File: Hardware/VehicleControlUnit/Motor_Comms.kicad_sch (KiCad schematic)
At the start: 47 parts

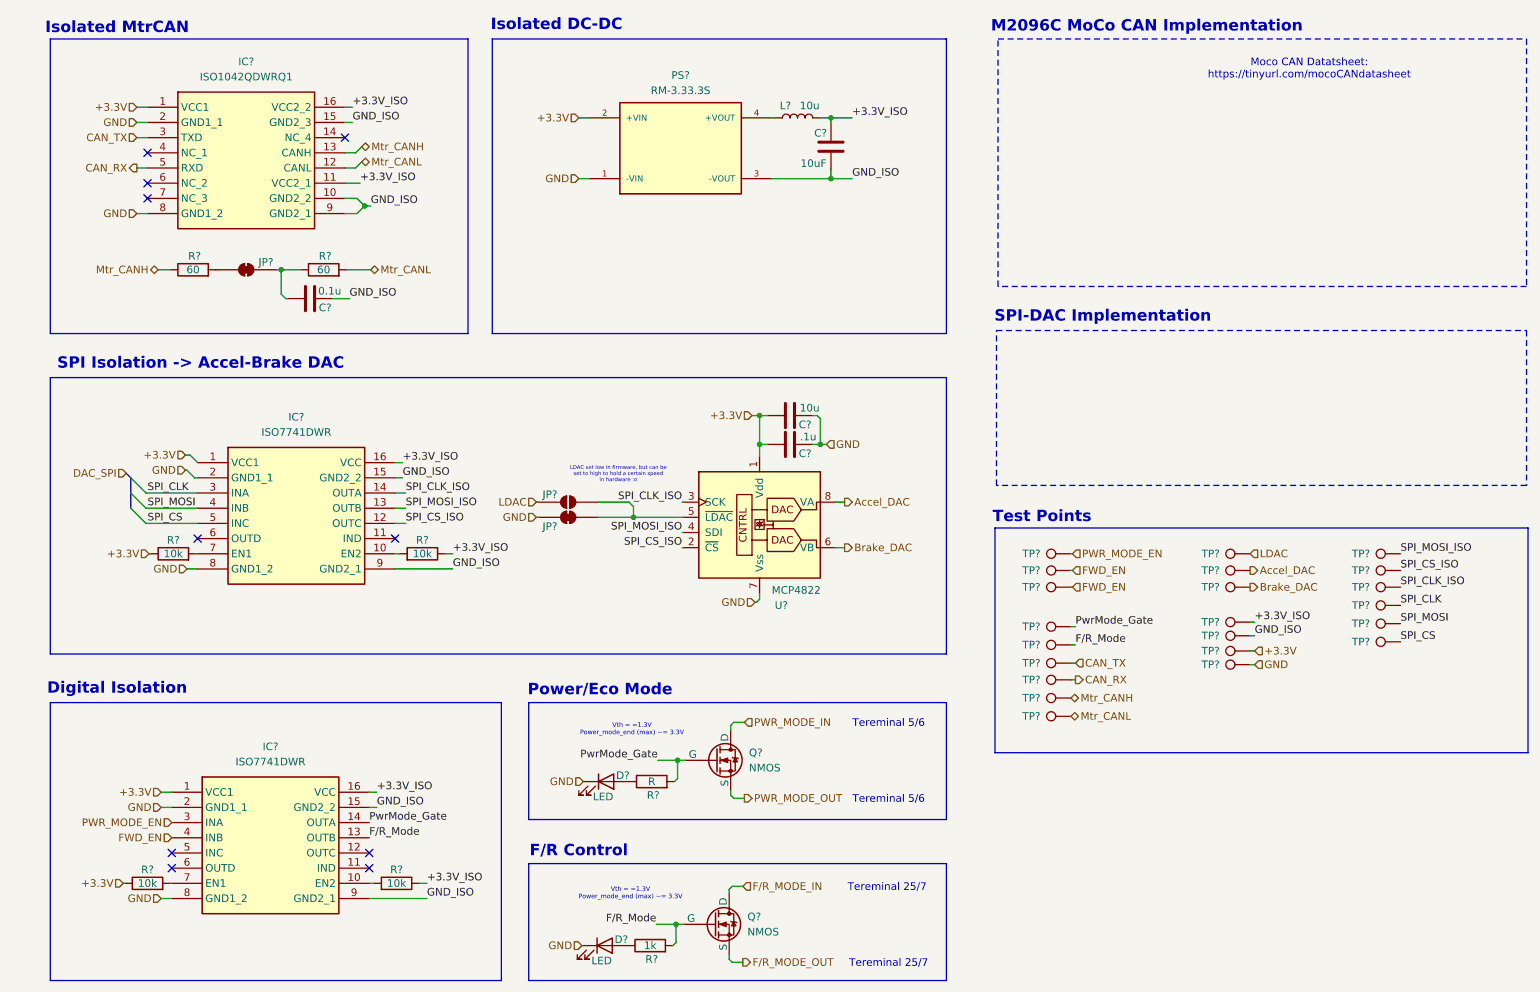
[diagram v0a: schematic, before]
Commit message: VCU more like diddle-u, mika time
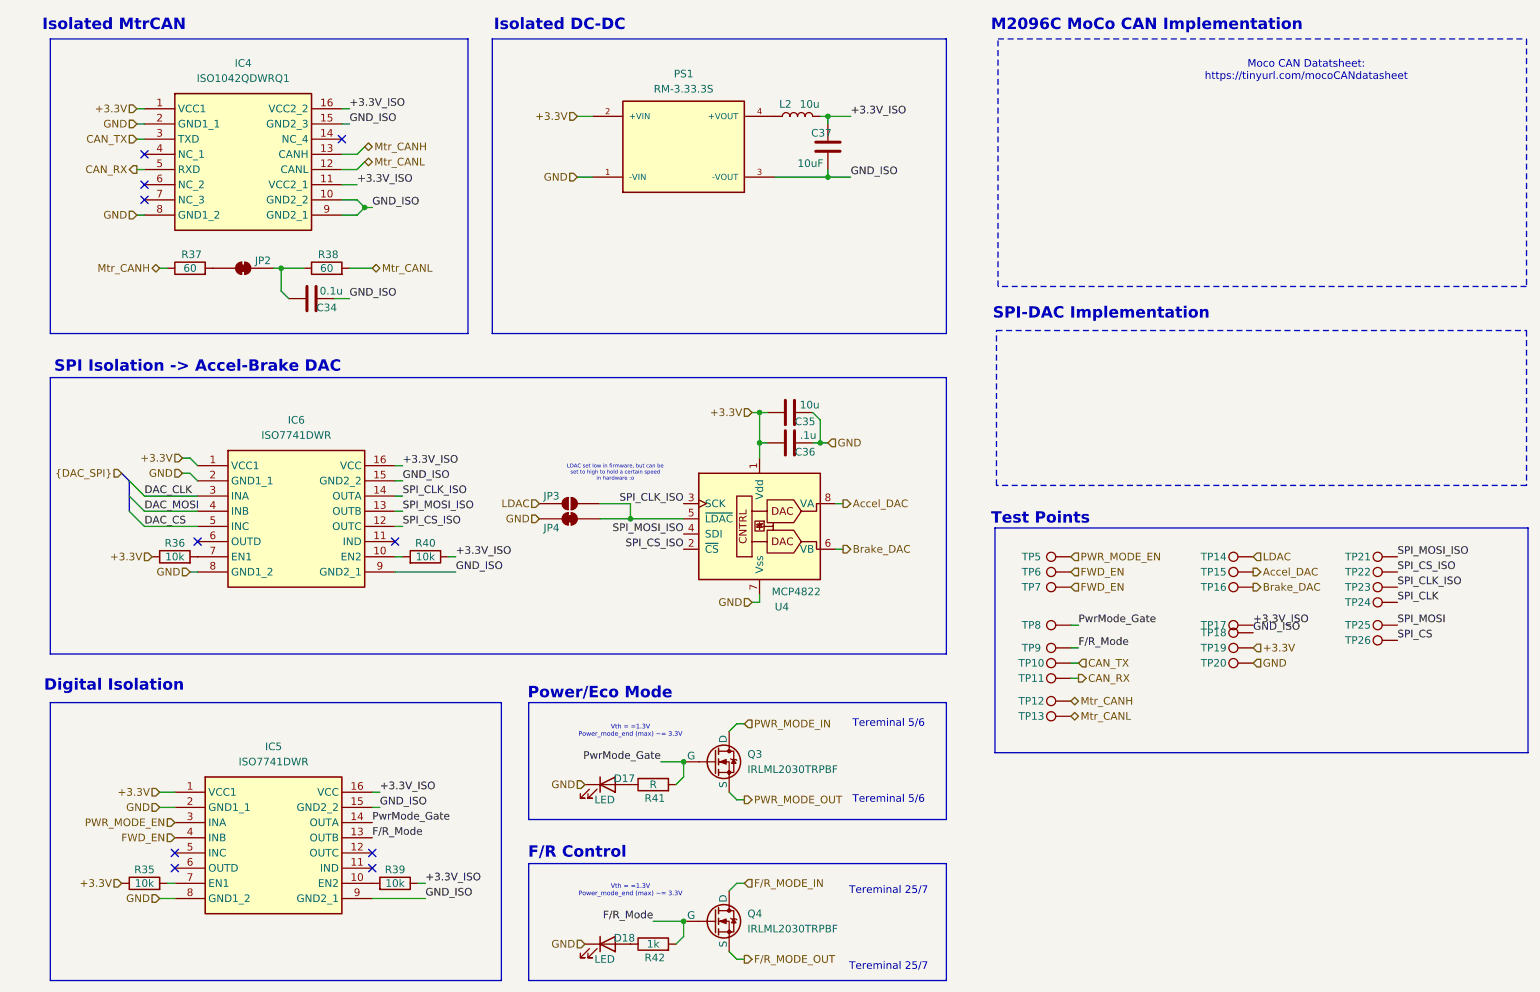
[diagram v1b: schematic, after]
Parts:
- removed Q?: NMOS, symbol Simulation_SPICE:NMOS
- added Q3: IRLML2030TRPBF, symbol Simulation_SPICE:NMOS
- Q4: renamed from Q?; value NMOS -> IRLML2030TRPBF; P/N (none) -> IRLML2030TRPBF
- gave numbers to parts that had none: 45
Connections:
- net PWR_MODE_IN: now also Q3.1 (D)
- net PWR_MODE_OUT: now also Q3.3 (S)
- net PwrMode_Gate: now also Q3.2 (G)
- net SPI_CLK: no longer IC6.3 (INA)
- net SPI_CS: no longer IC6.5 (INC)
- net SPI_MOSI: no longer IC6.4 (INB)
- new net DAC_CLK: IC6.3 (INA)
- new net DAC_CS: IC6.5 (INC)
- new net DAC_MOSI: IC6.4 (INB)
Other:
- moved on the sheet: C35, C37, D17, D18, IC4, IC5, IC6, JP2, PS1, Q4, R35, R36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
